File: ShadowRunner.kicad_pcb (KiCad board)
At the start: 2 copper layers, 69 parts, among them J1 micro JST SH, J2 GRPB052VWQS-RC, J3 SIM_Card, J4 MM8130-2600, J5 U.FL-R-SMT-1, Q1 DMN65D8L, Q2 DMN65D8L, U1 LM1117-ADJ, U2 USB-C, U3 LM1117-ADJ, U4 LIS2DS12, U5 SKY65943-11, U6 CM1402, U7 nRF9160, U8 PTS645SM43SMTR92, U9 PTS645SM43SMTR92

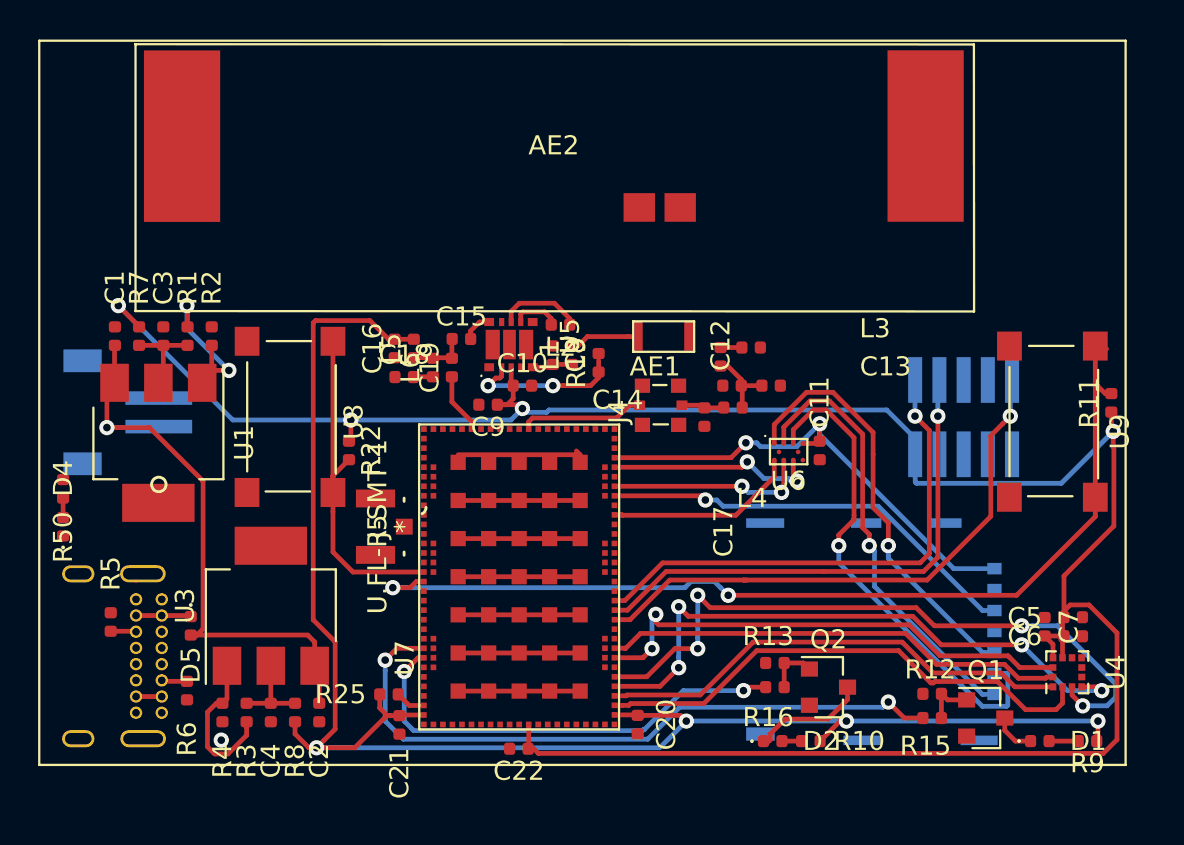
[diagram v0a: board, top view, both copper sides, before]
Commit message: All connections made
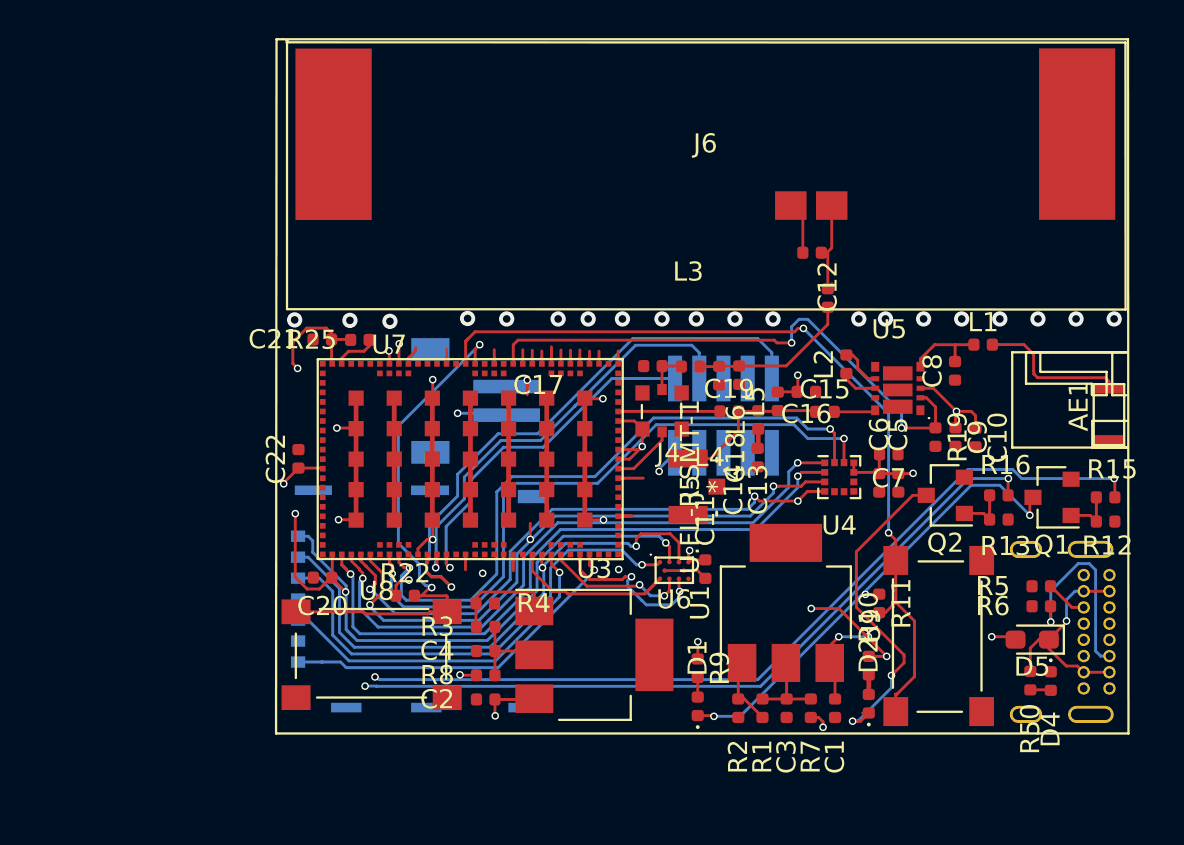
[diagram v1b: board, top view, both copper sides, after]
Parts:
- removed AE2: Antenna_Chip, MyLibs:PCS.06.A
- added J6: PCS.06.A, MyLibs:PCS.06.A, F.Cu at (134.2, 101.4)
- D5: value DIODE -> PMEG2020EPK,315; footprint Diode_SMD:D_0402_1005Metric -> MyLibs:D_0603_1608Metric_Pad1.05x0.95mm_HandSolder
- moved D4 52.5 mm to (152.3, 130.1), turned to 270 degrees
- moved R50 51.7 mm to (151.2, 130.1)
- moved U2 49.7 mm to (153.2, 127.5)
- moved R5 48.9 mm to (151.8, 125.1), turned to 180 degrees
- moved R6 45.0 mm to (151.8, 126.2), turned to 180 degrees
- moved D5 44.2 mm to (151.3, 127.9), turned to 180 degrees
- moved C1 42.5 mm to (141.0, 131.5), turned to 270 degrees
- moved R7 40.3 mm to (139.7, 131.5), turned to 90 degrees
- moved C3 38.1 mm to (138.5, 131.5), turned to 270 degrees
- moved J3 37.5 mm to (112.5, 128.8), turned to 270 degrees
- moved R1 35.9 mm to (137.2, 131.5), turned to 270 degrees
- moved U1 34.0 mm to (138.4, 126.0), turned to 90 degrees
- moved R2 33.8 mm to (135.9, 131.5), turned to 270 degrees
- moved C9 24.6 mm to (147.3, 117.3), turned to 270 degrees
- moved C10 23.9 mm to (148.4, 117.3), turned to 270 degrees
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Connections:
- C16 pad 2: +3V3 -> +1V8
- L5 pad 2: +3V3 -> +1V8
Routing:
- net VBUS: track 31.6 -> 79.8 mm, vias 1 -> 5
- net Net-(R16-Pad2): track 24.0 -> 59.5 mm, vias 2 -> 3
- net GND: track 46.7 -> 79.6 mm, vias 1 -> 32
- net Net-(R15-Pad2): track 35.3 -> 65.4 mm, vias 2 -> 3
- net +3V3: track 88.0 -> 58.0 mm, vias 4 -> 7
- net Net-(D1-Pad1): track 2.24 -> 24.1 mm, vias 0 -> 2
- net GPS_EN: track 7.95 -> 29.2 mm
- net +1V8: track 124.4 -> 108.6 mm, vias 4 -> 8
- net Net-(D2-Pad1): track 6.15 -> 17.5 mm, vias 0 -> 2
- net Net-(R22-Pad2): track 18.3 -> 28.1 mm, vias 0 -> 2
- net ACC_INT2: track 24.3 -> 33.9 mm, vias 0 -> 2
- net Net-(R6-Pad1): track 1.34 -> 10.6 mm, vias 0 -> 1
- net Net-(R11-Pad2): track 51.5 -> 43.5 mm
- net ACC_INT1: track 26.3 -> 34.2 mm
- net ACC_CLK: track 25.1 -> 32.9 mm, vias 0 -> 2
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- added copper zone on In1.Cu, net GND
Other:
- copper layers 2 -> 4
- rule trace_min: 0.2 -> 0.1524
- rule via_min_drill: 0.3 -> 0.24892
- rule via_min_size: 0.4 -> 0.3048
